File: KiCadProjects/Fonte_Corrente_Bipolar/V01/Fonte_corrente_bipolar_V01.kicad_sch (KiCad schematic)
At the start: 50 parts, among them J1 alimentacao analogica, J2 sinais analogicos, J3 comunicacao / sinais digitais, J4 SinA | Sin1, J5 SinB | Sin2, J7 +3.3V | +5.0V, U1-INA-I1 INA128, U1-howland1 AD828AN, U2-INA-I2 INA128, U3-cond1 AD828AN

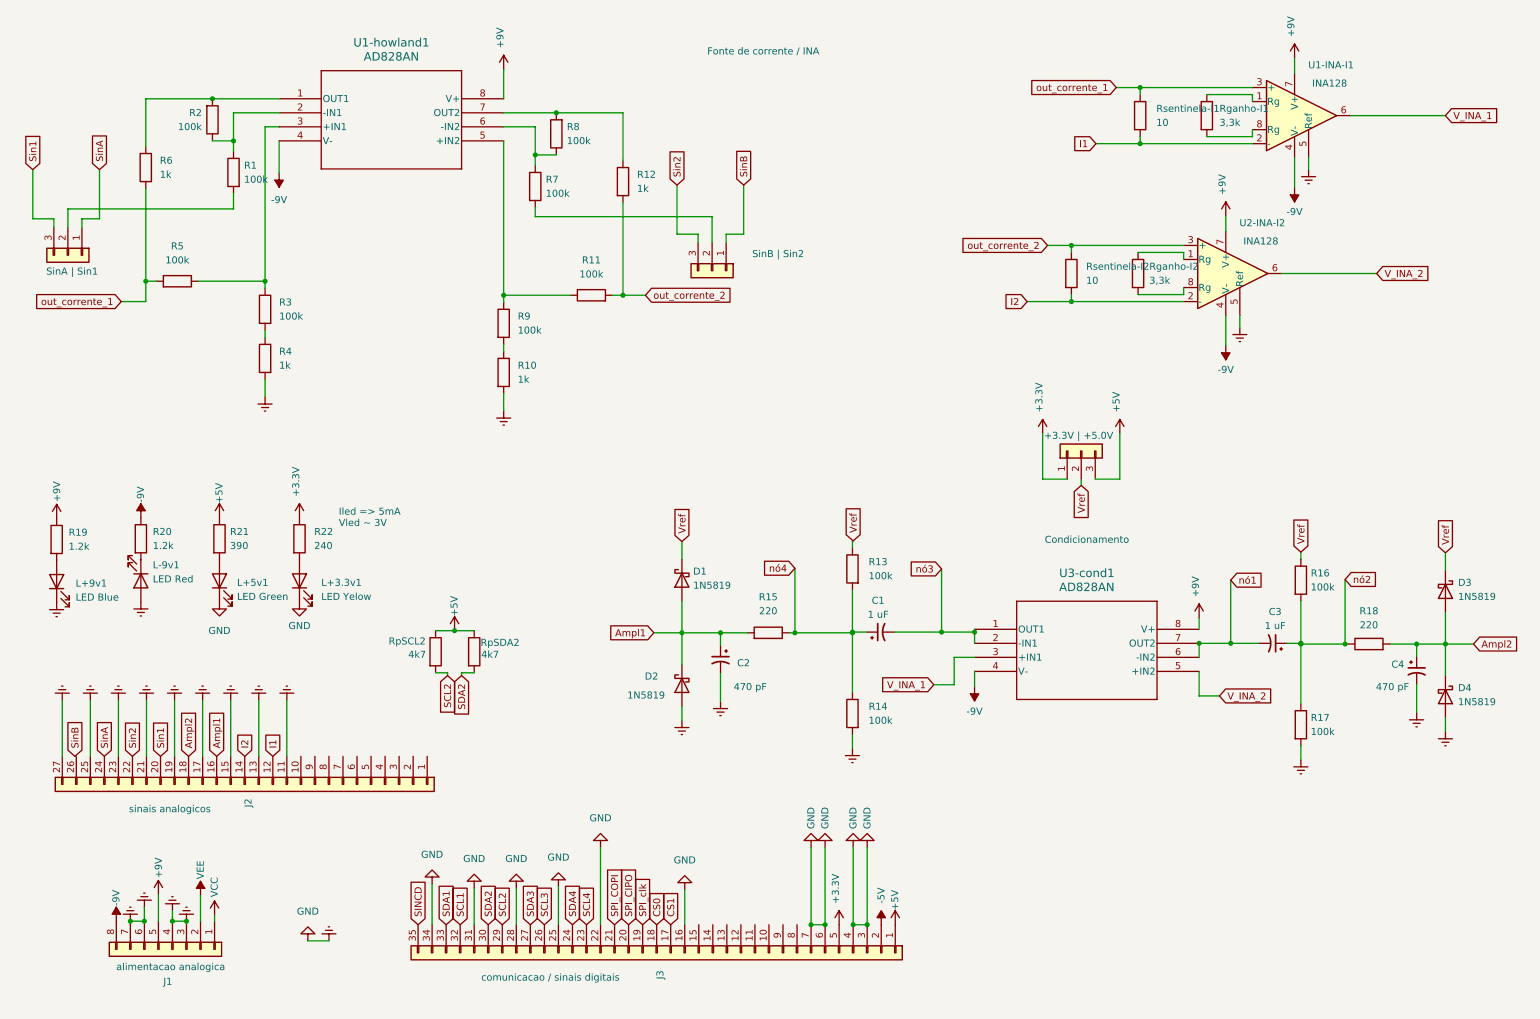
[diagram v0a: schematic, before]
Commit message: temp
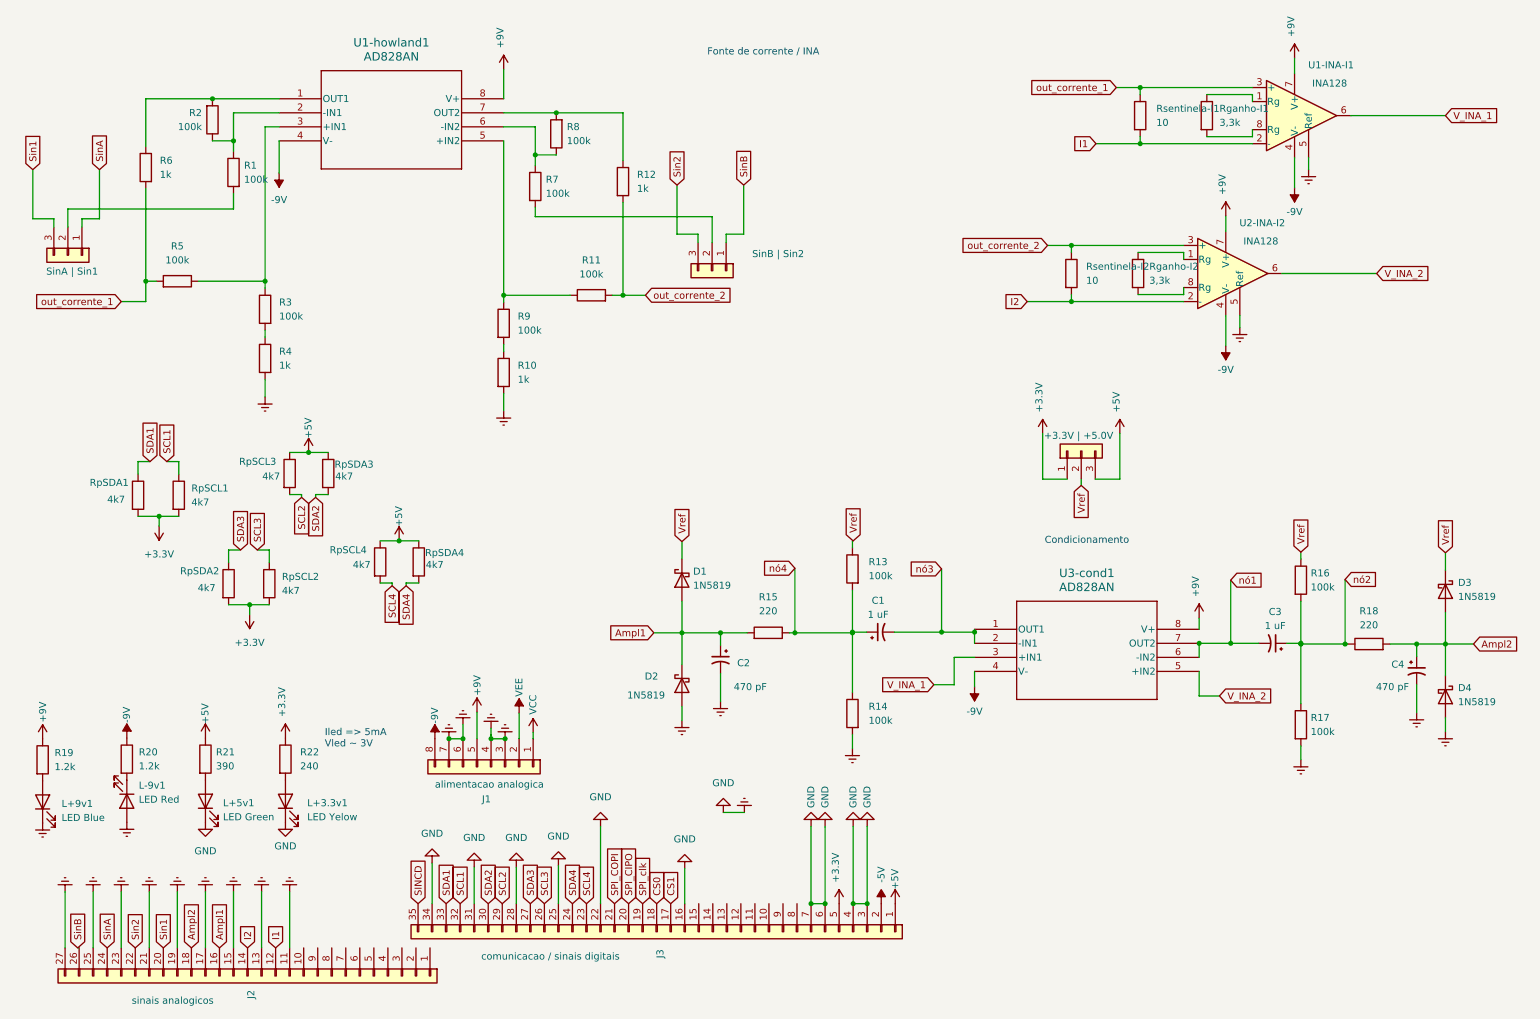
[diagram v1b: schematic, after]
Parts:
- added RpSCL1, RpSCL3, RpSCL4, RpSDA1, RpSDA3, RpSDA4: 4k7, Resistor_THT:R_Axial_DIN0207_L6.3mm_D2.5mm_P7.62mm_Horizontal, symbol Device:R
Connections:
- net +3.3V: now also RpSCL2.2, RpSDA2.2, RpSCL1.2, RpSDA1.2
- net +5V: now also RpSCL3.1, RpSCL4.1, RpSDA3.1, RpSDA4.1; no longer RpSCL2.1, RpSDA2.1
- net SCL1: now also RpSCL1.1
- net SCL2: now also RpSCL3.2; no longer RpSCL2.2
- net SCL3: now also RpSCL2.1
- net SCL4: now also RpSCL4.2
- net SDA1: now also RpSDA1.1
- net SDA2: now also RpSDA3.2; no longer RpSDA2.2
- net SDA3: now also RpSDA2.1
- net SDA4: now also RpSDA4.2
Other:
- moved on the sheet: J1, J2, J3, L+3.3v1, L+5v1, L+9v1, L-9v1, R19, R20, R21, R22

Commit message: em producao
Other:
- title: Fonte de corrente monopolar -> Fonte de corrente bipolar
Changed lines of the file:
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@@
   (paper "A4")
   (title_block
-    (title "Fonte de corrente monopolar")
-    (date "2023-07-14")
-    (rev "v02")
+    (title "Fonte de corrente bipolar")
+    (date "2024-06-06")
+    (rev "v01")
     (company "EITduino")
     (comment 1 "Autor: Gustavo Pinheiro")
-    (comment 2 "Placa de face dupla 90x100 mm")
+    (comment 2 "Placa de face dupla 100x100 mm")
     (comment 3 "Barramento V04")
     (comment 4 "Howland aperfeicoada")
